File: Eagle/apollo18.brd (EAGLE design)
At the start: 90.6 x 102.5 mm, 29 parts, among them IC1 L298, IC2 7808T, IC3 7808T, IC4 7805T, IC5 7805T, IC6 7805T

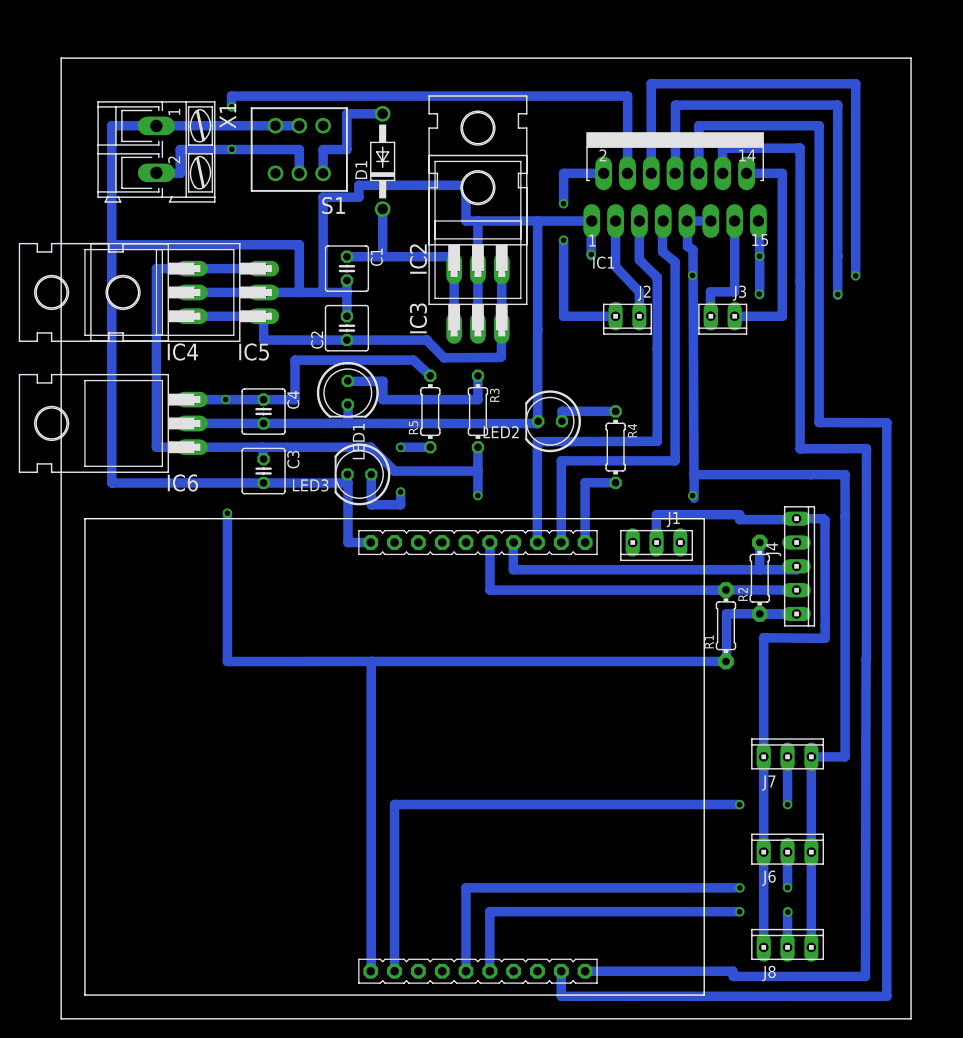
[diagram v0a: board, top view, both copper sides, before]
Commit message: Update Eagle CAD PCB files
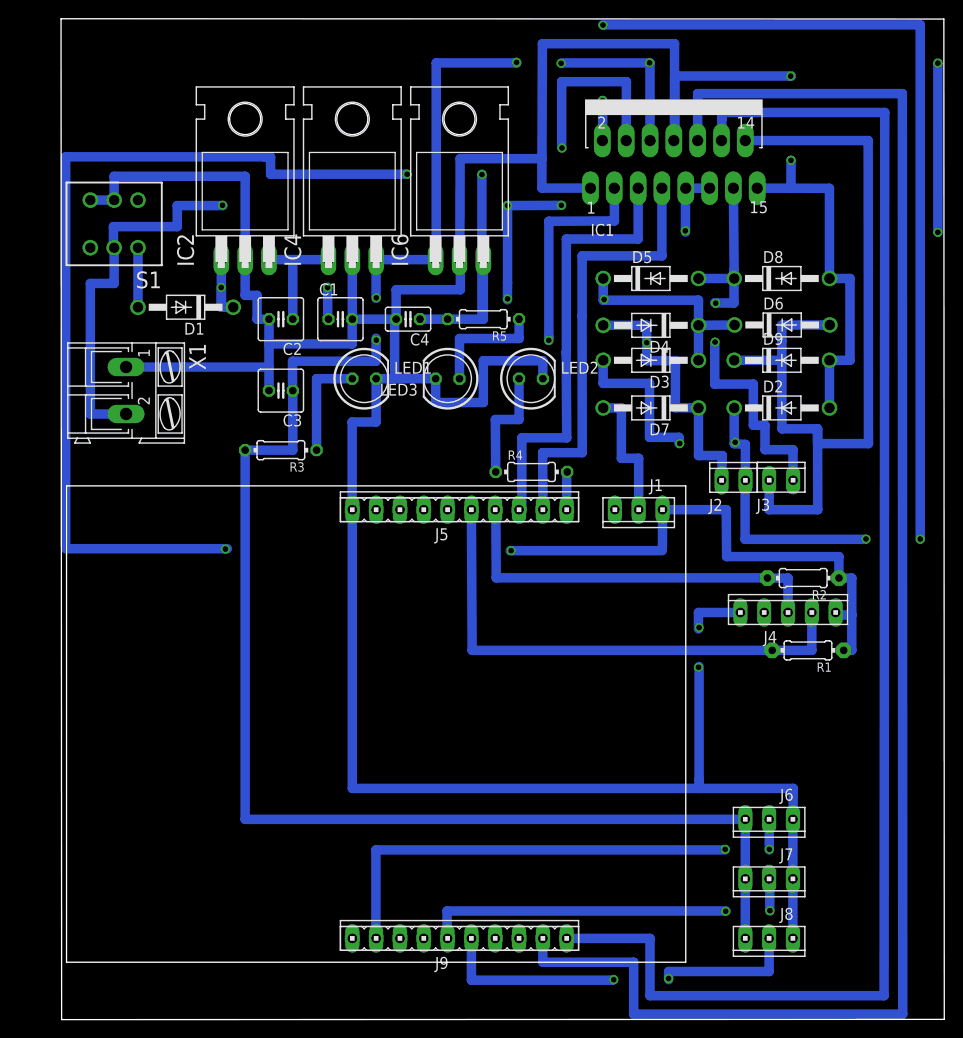
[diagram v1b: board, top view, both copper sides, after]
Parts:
- removed IC3: 7808T, linear:TO220H
- removed IC5: 7805T, linear:TO220H
- added D2, D3, D4, D5, D6, D7, D8, D9: 1N4004, diode:DO41-10
- added J5, J9: (no value), con-amp:10X10MTA
- C4: device rcl:C025-050X050 -> rcl:C025-025X050
- moved IC6 47.5 mm to (42.5, 91.1), turned to 0 degrees
- moved IC4 30.5 mm to (31.1, 91.1), turned to 0 degrees
- moved D1 26.1 mm to (13.3, 75.9), turned to 180 degrees
- moved X1 25.9 mm to (6.92, 67.0)
- moved IC2 24.8 mm to (19.6, 91.1)
- moved R3 21.4 mm to (23.4, 60.6), turned to 180 degrees
- moved S1 21.3 mm to (5.65, 84.8)
- moved J2 20.8 mm to (71.7, 57.4), turned to 0 degrees
- moved J3 18.6 mm to (76.8, 57.4), turned to 0 degrees
- moved C4 18.3 mm to (37.0, 74.6), turned to 180 degrees
- moved LED3 13.9 mm to (41.2, 68.3)
- moved J7 13.2 mm to (75.5, 14.9), turned to 180 degrees
- moved R5 11.4 mm to (45.0, 74.6), turned to 180 degrees
- moved R4 9.36 mm to (50.2, 58.3), turned to 0 degrees
- moved R1 9.13 mm to (79.6, 39.3), turned to 180 degrees
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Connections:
- net +12V: now also D3.C, D4.C, D5.C, D6.C
- net +5V: no longer IC5.3
- net AN1: now also U$1.P1.3; no longer U$1.P1.0
- net AN2: now also U$1.P1.0; no longer U$1.P1.3
- net GND: now also D2.A, D7.A, D8.A, D9.A; no longer IC3.2, IC5.2
- net N$2: now also D2.C, D3.A
- net N$3: now also D4.A, D7.C
- net N$4: now also D5.A, D8.C
- net N$5: now also D6.A, D9.C
- net N$6: no longer IC3.1
- net N$8: no longer IC3.3, IC5.1
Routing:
- net N$2: track 21.2 -> 139.3 mm
- net N$5: track 24.1 -> 94.5 mm
- net N$3: track 11.2 -> 52.4 mm
- net N$8: track 45.9 -> 12.7 mm
- net +3.3V: track 117.8 -> 150.3 mm
- net N$33: track 31.2 -> 0.00 mm
- net N$4: track 12.8 -> 42.8 mm
- net +12V: track 72.0 -> 99.1 mm
- net AN1: track 59.7 -> 36.2 mm
- net SDA: track 37.8 -> 55.3 mm
- net IN4: track 137.2 -> 154.6 mm
- net N$10: track 0.00 -> 17.2 mm, vias 1 -> 0
- net N$14: track 0.00 -> 16.2 mm, vias 1 -> 0
- net IN3: track 155.3 -> 171.5 mm
- net +5V: track 226.9 -> 214.5 mm
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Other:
- board size 90.6 x 102.5 mm -> 94.2 x 106.7 mm
